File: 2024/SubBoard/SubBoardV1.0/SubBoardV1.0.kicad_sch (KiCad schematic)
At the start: 18 parts, among them J1 Conn_01x02_Socket, J10 Conn_01x02_Socket, J11 Conn_01x03_Socket, J12 Conn_01x02_Socket, J13 Conn_01x02_Socket, J14 Conn_01x06_Socket, J15 Conn_01x06_Socket, J16 Conn_01x12_Socket, J2 Conn_01x02_Socket, J3 Conn_01x02_Socket, J4 Conn_01x02_Socket, J5 Conn_01x02_Socket, J6 Conn_01x02_Socket, J7 Conn_01x02_Socket, J8 Conn_01x02_Socket, J9 Conn_01x02_Socket

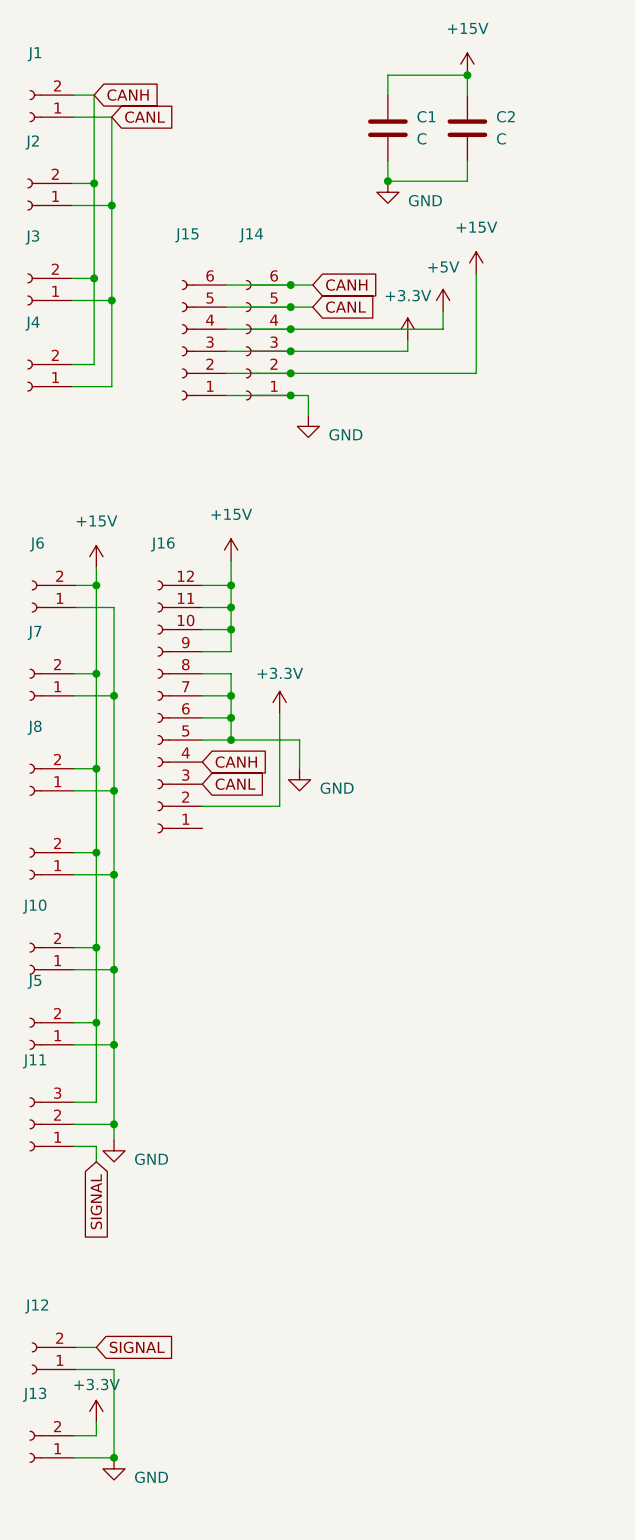
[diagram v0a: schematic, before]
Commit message: add Kick&Sub
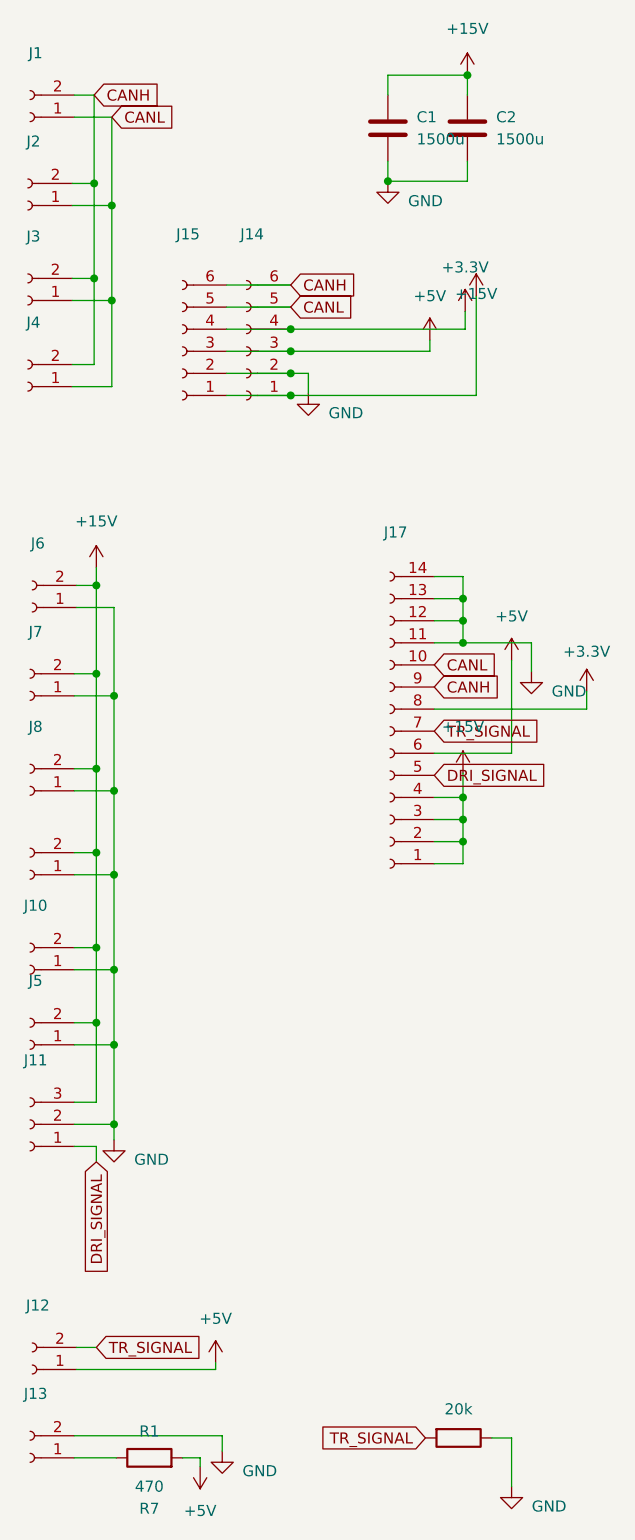
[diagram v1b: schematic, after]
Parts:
- removed J16: Conn_01x12_Socket, Connector_PinHeader_2.54mm:PinHeader_2x06_P2.54mm_Vertical, symbol Connector:Conn_01x12_Socket
- added J17: Conn_01x14_Socket, Connector_PinHeader_2.54mm:PinHeader_2x07_P2.54mm_Vertical, symbol Connector:Conn_01x14_Socket
- added R1: 20k, Resistor_SMD:R_0603_1608Metric, symbol Device:R
- added R7: 470, Resistor_SMD:R_0603_1608Metric, symbol Device:R
- C1, C2: value C -> 1500u; footprint Capacitor_SMD:CP_Elec_10x10 -> Capacitor_THT:CP_Radial_D12.5mm_P5.00mm
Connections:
- net +15V: now also J14.1 (Pin_1), J15.1 (Pin_1), J17.1 (Pin_1), J17.2 (Pin_2), J17.3 (Pin_3), J17.4 (Pin_4); no longer J14.2 (Pin_2), J15.2 (Pin_2)
- net +3.3V: now also J14.4 (Pin_4), J15.4 (Pin_4), J17.8 (Pin_8); no longer J13.2 (Pin_2), J14.3 (Pin_3), J15.3 (Pin_3)
- net +5V: now also J12.1 (Pin_1), J14.3 (Pin_3), J15.3 (Pin_3), J17.6 (Pin_6), R7.2; no longer J14.4 (Pin_4), J15.4 (Pin_4)
- net CANH: now also J17.9 (Pin_9)
- net CANL: now also J17.10 (Pin_10)
- net GND: now also J13.2 (Pin_2), J14.2 (Pin_2), J15.2 (Pin_2), J17.11 (Pin_11), J17.12 (Pin_12), J17.13 (Pin_13), J17.14 (Pin_14), R1.1; no longer J12.1 (Pin_1), J13.1 (Pin_1), J14.1 (Pin_1), J15.1 (Pin_1)
- net SIGNAL renamed DRI_SIGNAL
- net DRI_SIGNAL: now also J17.5 (Pin_5); no longer J12.2 (Pin_2)
- new net: J13.1 (Pin_1), R7.1
- new net TR_SIGNAL: J12.2 (Pin_2), J17.7 (Pin_7), R1.2
